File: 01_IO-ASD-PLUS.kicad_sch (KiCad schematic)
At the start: 2 parts

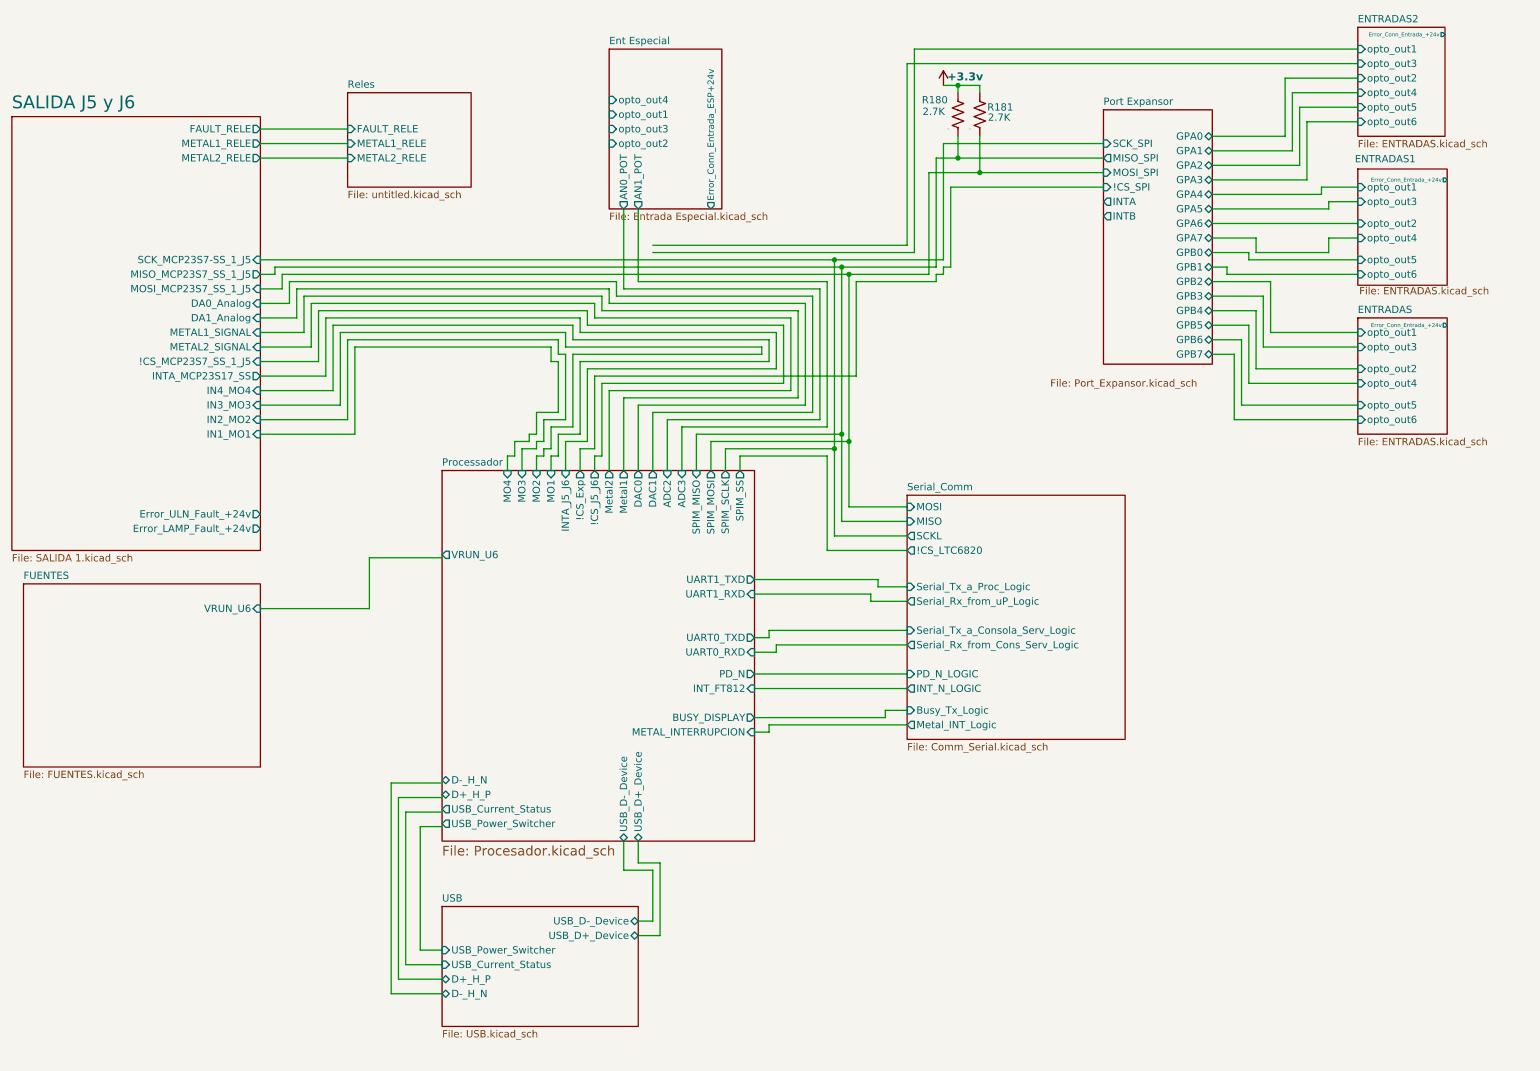
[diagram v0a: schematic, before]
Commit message: pcb 18 may 26
 falta poner la fuente de +12/ ya esta casi todo
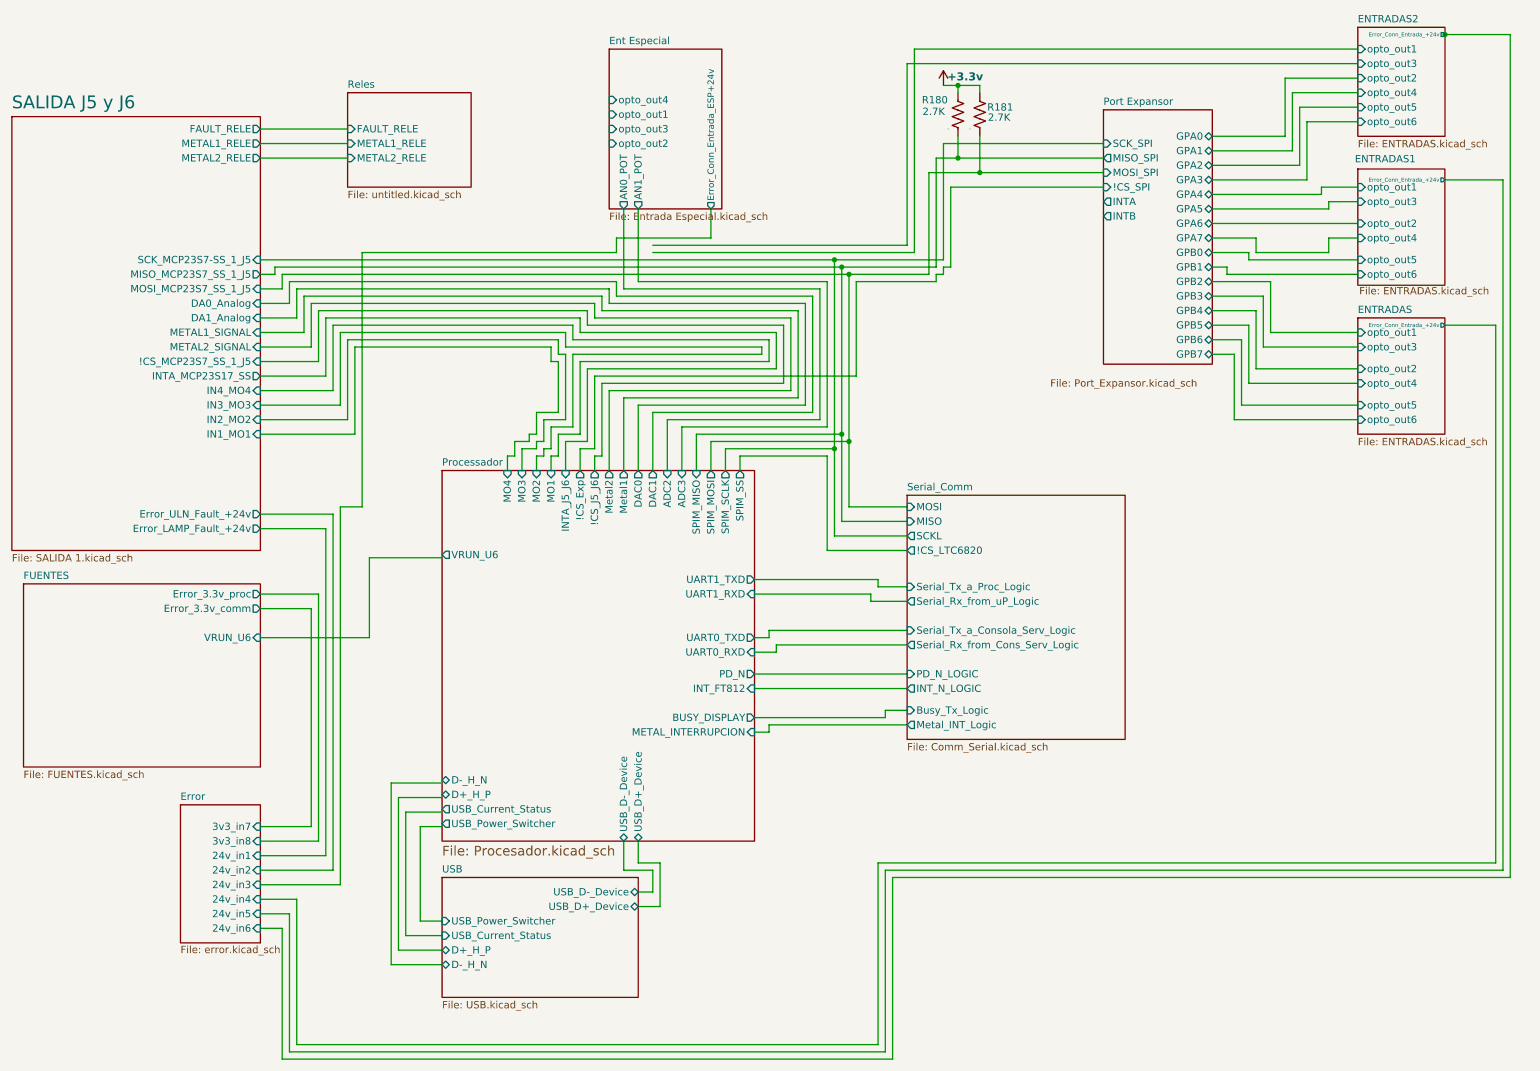
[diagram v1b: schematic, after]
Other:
- added sheet Error (error.kicad_sch)
- sheet FUENTES ports: added Error_3.3v_comm, Error_3.3v_proc; removed none
